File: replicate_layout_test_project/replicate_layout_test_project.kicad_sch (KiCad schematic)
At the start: 1 part, among them U101 TMS320F28027DA

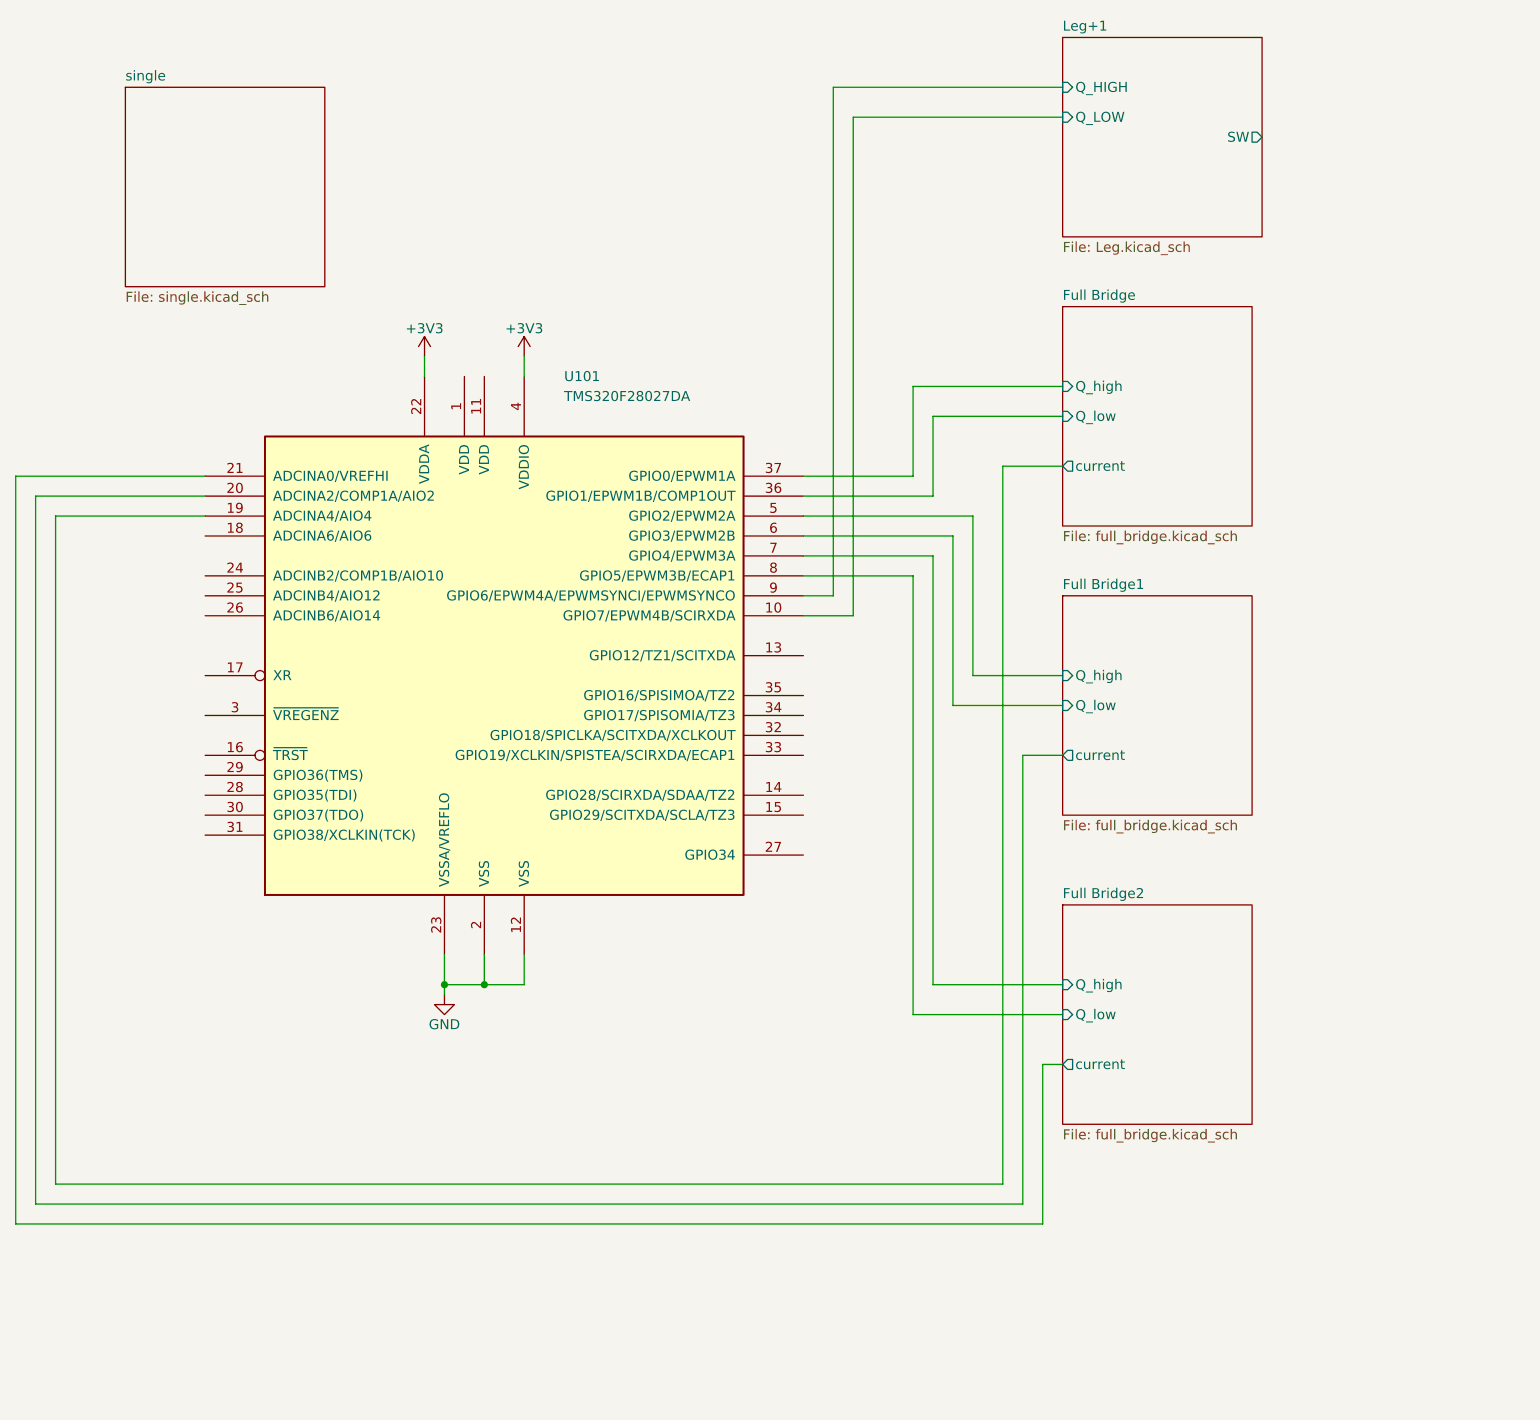
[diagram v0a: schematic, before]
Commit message: updated test project
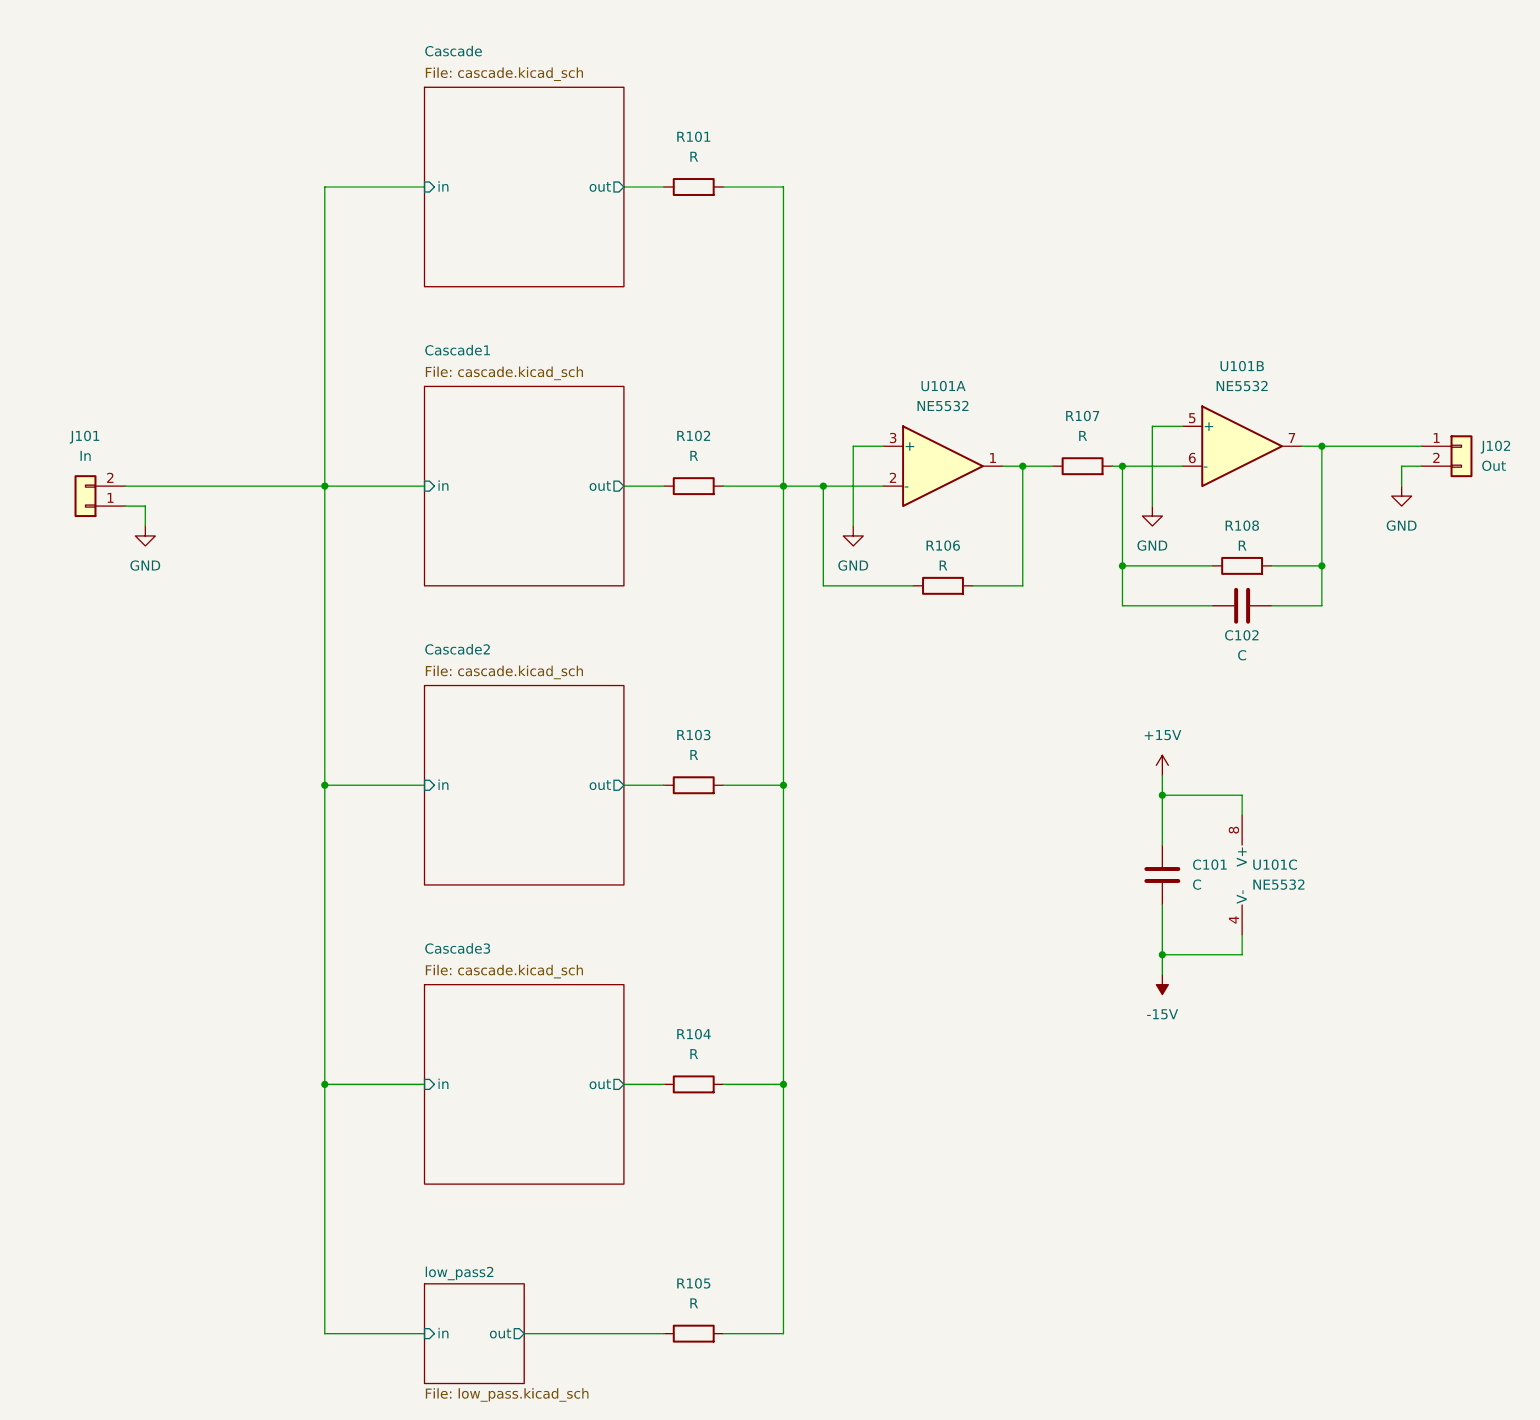
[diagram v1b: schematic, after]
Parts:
- removed U101: TMS320F28027DA, Package_SO:TSSOP-38_4.4x9.7mm_P0.5mm, symbol ICs:TMS320F28027DA
- added C101, C102: C, Capacitor_SMD:C_1206_3216Metric, symbol Device:C
- added J101: In, Connector_PinHeader_2.54mm:PinHeader_1x02_P2.54mm_Vertical, symbol Connector_Generic:Conn_01x02
- added J102: Out, Connector_PinHeader_2.54mm:PinHeader_1x02_P2.54mm_Vertical, symbol Connector_Generic:Conn_01x02
- added R101, R102, R103, R104, R105, R106, R107, R108: R, Resistor_SMD:R_1206_3216Metric, symbol Device:R
- added U101: NE5532, Package_SO:SOIC-8_5.23x5.23mm_P1.27mm, symbol Amplifier_Operational:NE5532
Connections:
- net GND: now also J101.1 (Pin_1), J102.2 (Pin_2), U101.3 (+), U101.5 (+)
- new net: R106.2, R107.1, U101.1
- new net: C102.2, R107.2, R108.1, U101.6 (-)
- new net: R101.2, R102.2, R103.2, R104.2, R105.2, R106.1, U101.2 (-)
- new net: C102.1, J102.1 (Pin_1), R108.2, U101.7
- new net +15V: C101.1, U101.8 (V+)
- new net -15V: C101.2, U101.4 (V-)
- new net Cascade/in: J101.2 (Pin_2)
- new net Cascade/out: R101.1
- new net Cascade1/out: R102.1
- new net Cascade2/out: R103.1
- new net Cascade3/out: R104.1
- new net low_pass2/out: R105.1
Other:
- removed sheet Full Bridge
- removed sheet Full Bridge1
- removed sheet Full Bridge2
- removed sheet Leg+1
- removed sheet single
- added sheet Cascade (cascade.kicad_sch)
- added sheet Cascade1 (cascade.kicad_sch)
- added sheet Cascade2 (cascade.kicad_sch)
- added sheet Cascade3 (cascade.kicad_sch)
- added sheet low_pass2 (low_pass.kicad_sch)
